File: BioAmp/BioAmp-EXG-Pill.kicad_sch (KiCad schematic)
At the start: 42 parts, among them IC3 MAX1169BEUD+, J2 Conn_01x04_Pin, J3 Conn_01x04_Pin, J4 522710469, U1 TL074HIPWR

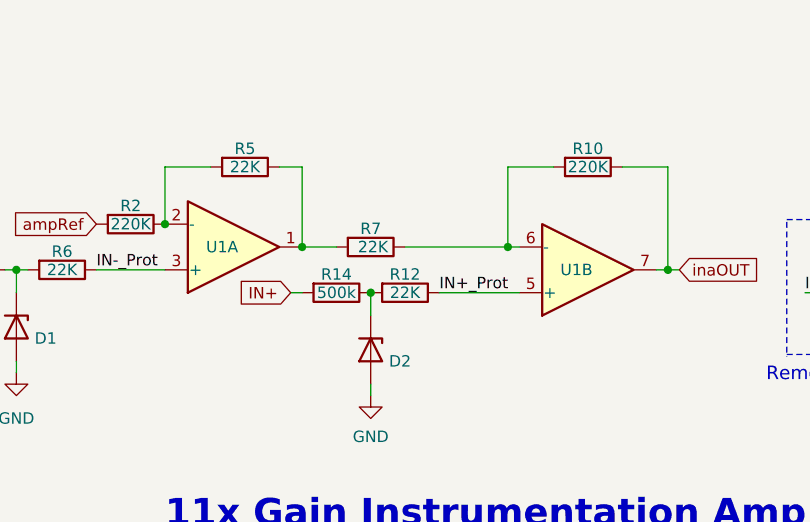
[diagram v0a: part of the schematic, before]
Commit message: Did component placement
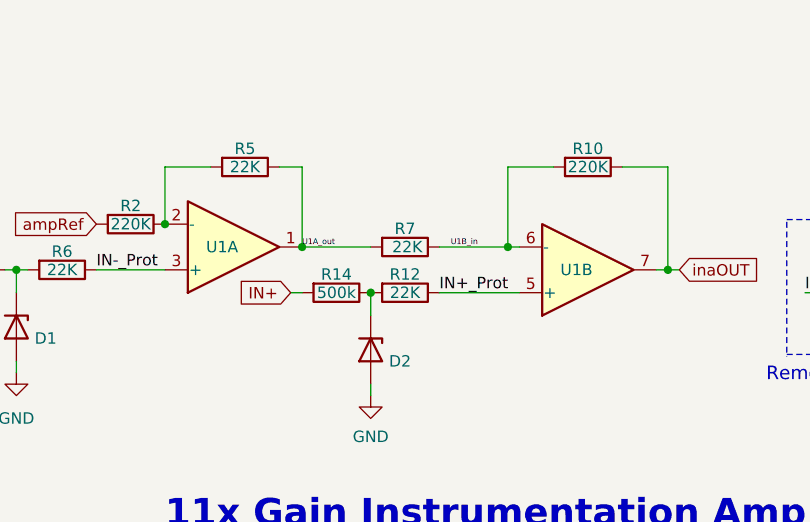
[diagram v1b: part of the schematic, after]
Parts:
- C10, C11, C9: footprint Capacitor_SMD:C_0603_1608Metric_Pad1.08x0.95mm_HandSolder -> Capacitor_SMD:C_0402_1005Metric
- J4: footprint CON_522710469_MOL -> FPC_Connector:CON_522710469_MOL
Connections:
- net U1B_in: now reaches R10.2, R7.1, U1.6 (-)
- net U1A_out: now reaches R5.1, R7.2, U1.1
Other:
- moved on the sheet: R7
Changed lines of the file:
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@@
 	)
 	(junction
-		(at 212.09 92.71)
+		(at 95.25 38.1)
 		(diameter 0)
 		(color 0 0 0 0)
 	)
 	(junction
-		(at 190.5 20.32)
+		(at 212.09 92.71)
 		(diameter 0)
 		(color 0 0 0 0)
 	)
 	(junction
-		(at 80.01 43.18)
+		(at 190.5 20.32)
 		(diameter 0)
 		(color 0 0 0 0)
 	)
 	(junction
-		(at 180.34 20.32)
+		(at 80.01 43.18)
 		(diameter 0)
 		(color 0 0 0 0)
 	)
 	(junction
-		(at 95.25 38.1)
+		(at 180.34 20.32)
 		(diameter 0)
 		(color 0 0 0 0)
@@
 	)
 	(junction
-		(at 72.39 38.1)
-		(diameter 0)
-		(color 0 0 0 0)
-	)
-	(junction
 		(at 40.64 40.64)
 		(diameter 0)
@@
 	)
 	(junction
+		(at 72.39 38.1)
+		(diameter 0)
+		(color 0 0 0 0)
+	)
+	(junction
 		(at 204.47 20.32)
 		(diameter 0)
@@
 	(wire
 		(pts
-			(xy 83.82 38.1) (xy 95.25 38.1)
+			(xy 87.63 38.1) (xy 95.25 38.1)
 		)
 		(stroke
@@
 	(wire
 		(pts
-			(xy 76.2 38.1) (xy 72.39 38.1)
+			(xy 80.01 38.1) (xy 72.39 38.1)
 		)
 		(stroke
@@
 		)
 	)
+	(label "U1A_out"
+		(at 72.39 38.1 0)
+		(effects
+			(font
+				(size 0.635 0.635)
+			)
+			(justify left bottom)
+		)
+	)
 	(label "IN-_Prot"
 		(at 49.53 40.64 0)
@@
 		)
 	)
+	(label "U1B_in"
+		(at 88.9 38.1 0)
+		(effects
+			(font
+				(size 0.635 0.635)
+			)
+			(justify left bottom)
+		)
+	)
 	(label "ADD0"
 		(at 254 22.86 0)
@@
 	(symbol
 		(lib_id "Device:R")
-		(at 80.01 38.1 270)
+		(at 83.82 38.1 270)
 		(unit 1)
 		(body_style 1)
@@
 		(dnp no)
 		(property "Reference" "R7"
-			(at 80.01 36.068 90)
+			(at 83.82 36.068 90)
 			(show_name no)
 			(do_not_autoplace no)
@@
 		)
 		(property "Value" "22K"
-			(at 80.264 38.1 90)
+			(at 84.074 38.1 90)
 			(show_name no)
 			(do_not_autoplace no)
@@
 		)
 		(property "Footprint" "Resistor_SMD:R_0603_1608Metric_Pad0.98x0.95mm_HandSolder"
-			(at 80.01 36.322 90)
+			(at 83.82 36.322 90)
 			(hide yes)
 			(show_name no)
@@
 		)
 		(property "Datasheet" ""
-			(at 80.01 38.1 0)
+			(at 83.82 38.1 0)
 			(hide yes)
 			(show_name no)
@@
 		)
 		(property "Description" ""
-			(at 80.01 38.1 0)
+			(at 83.82 38.1 0)
 			(show_name no)
 			(do_not_autoplace no)
@@
 			)
 		)
-		(property "Footprint" "Capacitor_SMD:C_0603_1608Metric_Pad1.08x0.95mm_HandSolder"
+		(property "Footprint" "Capacitor_SMD:C_0402_1005Metric"
 			(at 268.2748 21.59 0)
 			(hide yes)
@@
 			)
 		)
-		(property "Footprint" "Capacitor_SMD:C_0603_1608Metric_Pad1.08x0.95mm_HandSolder"
+		(property "Footprint" "Capacitor_SMD:C_0402_1005Metric"
 			(at 179.3748 21.59 0)
 			(hide yes)
@@
 			)
 		)
-		(property "Footprint" "Capacitor_SMD:C_0603_1608Metric_Pad1.08x0.95mm_HandSolder"
+		(property "Footprint" "Capacitor_SMD:C_0402_1005Metric"
 			(at 189.5348 21.59 0)
 			(hide yes)
@@
 			)
 		)
-		(property "Footprint" "CON_522710469_MOL"
+		(property "Footprint" "FPC_Connector:CON_522710469_MOL"
 			(at 229.87 140.97 0)
 			(hide yes)
